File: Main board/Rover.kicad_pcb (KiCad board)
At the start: 2 copper layers, 76.1 x 102.6 mm, 12 parts, among them J1 IN, J2 OUT, J3 Barrel_Jack_Switch, J4 MOTOR, J5 MOTOR, J6 MOTOR, J7 MOTOR, SW1 SW_DPDT_x2, U1 RASPBERRY_PI_4B_4GB

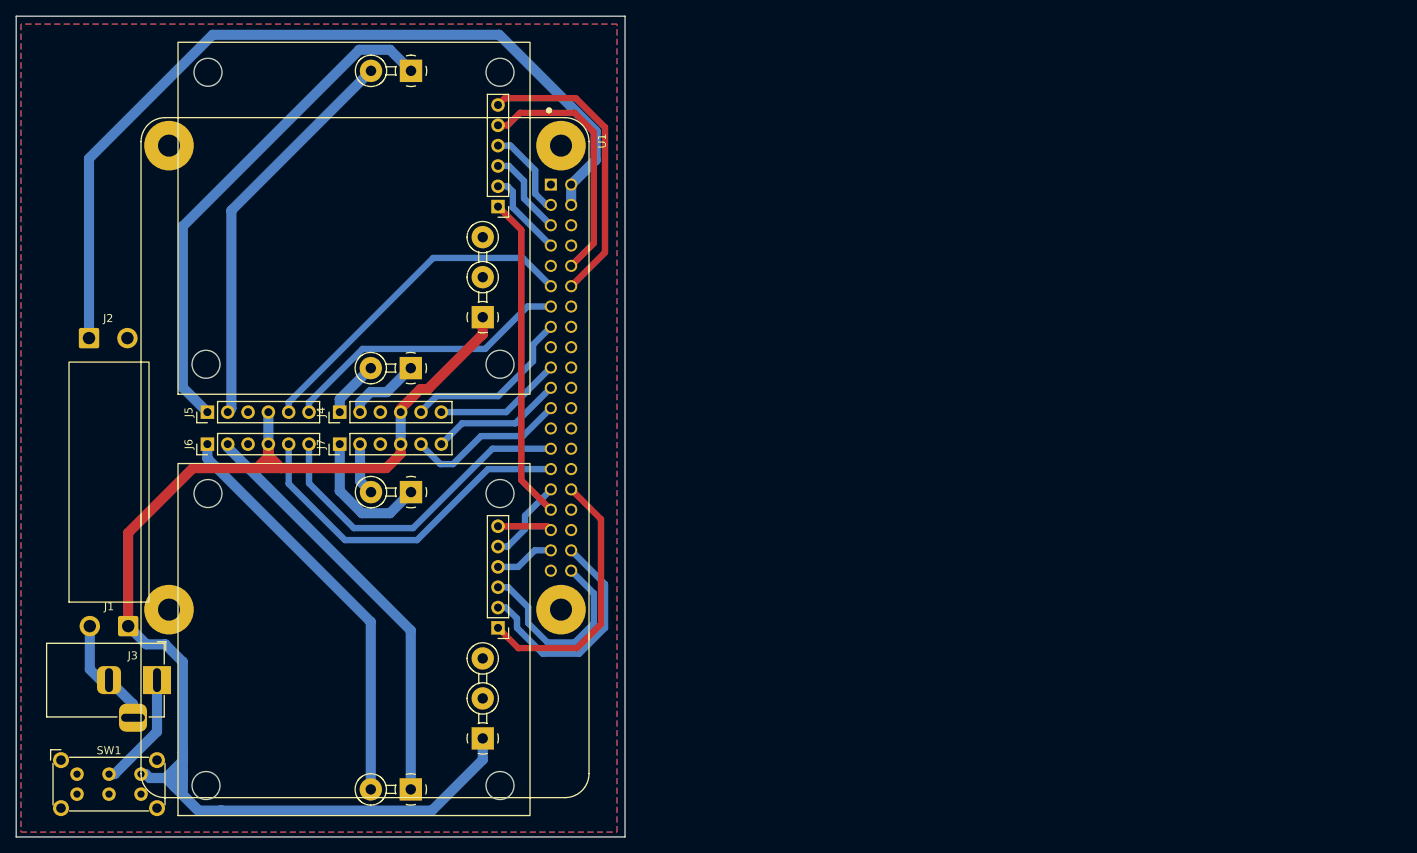
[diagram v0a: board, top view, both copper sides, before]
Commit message: updated pcb
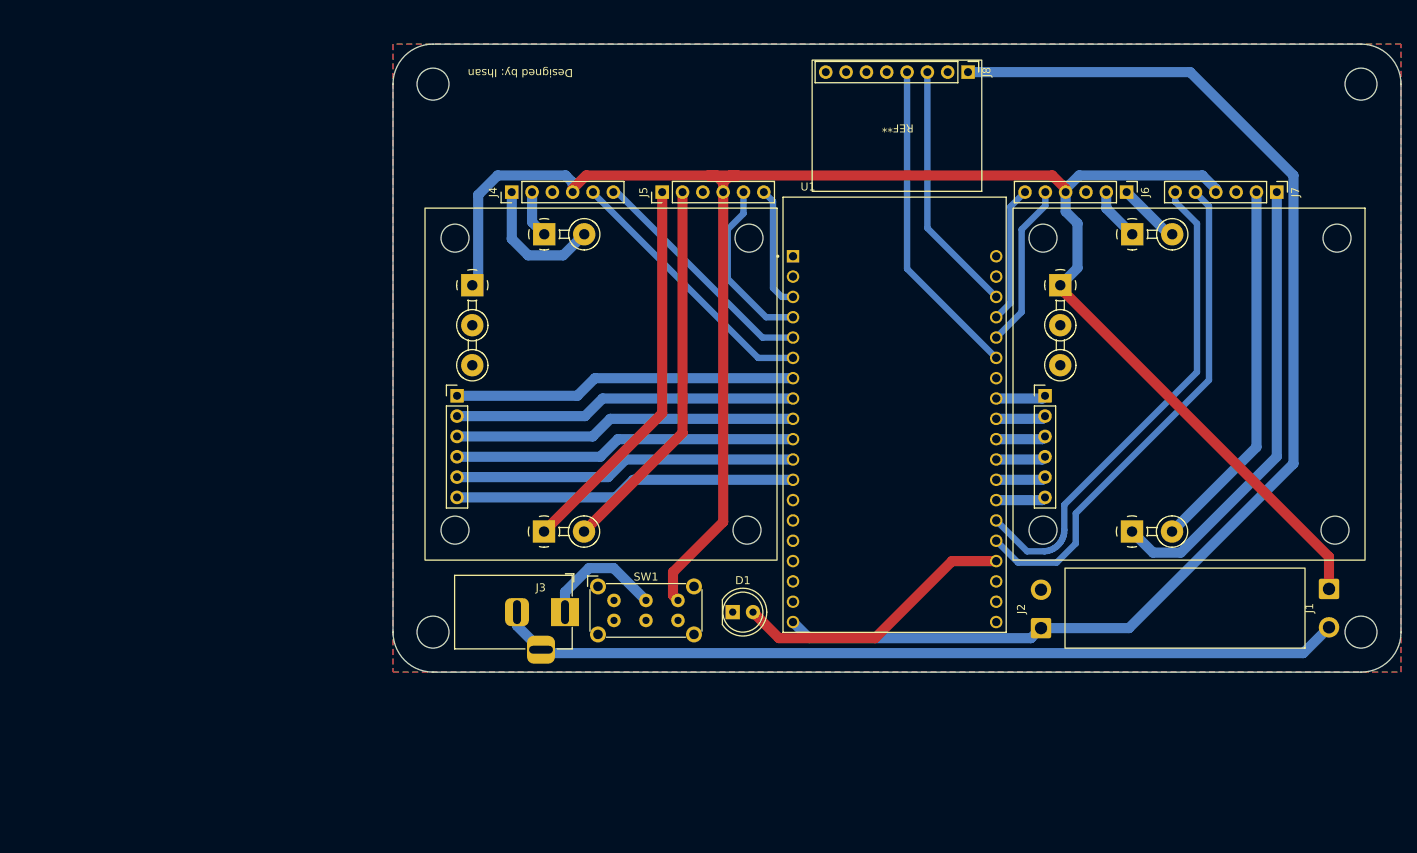
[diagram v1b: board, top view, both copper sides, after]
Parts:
- added D1: LED, LED_THT:LED_D5.0mm_Clear, F.Cu at (178.5, 120.5)
- added J8: IMU, Connector_PinHeader_2.54mm:PinHeader_1x08_P2.54mm_Vertical, F.Cu at (207.9, 53.0)
- added REF**: mpu 6050, module:mpu 6050, F.Cu at (199.1, 59.5)
- U1: value RASPBERRY_PI_4B_4GB -> ESP32-DEVKITC-32D; footprint RASPBERRY_PI_4B_4GB:MODULE_RASPBERRY_PI_4B_4GB -> Library:MODULE_ESP32-DEVKITC-32D
- moved J1 150.2 mm to (253.0, 117.6), turned to -90 degrees
- moved REF** 135.4 mm to (235.0, 120.0), turned to 180 degrees
- moved J2 124.4 mm to (217.0, 122.5), turned to 90 degrees
- moved J7 121.3 mm to (246.5, 68.0), turned to -90 degrees
- moved J6 119.1 mm to (227.7, 68.0), turned to -90 degrees
- moved U3 109.1 mm to (235.5, 92.0), turned to -90 degrees
- moved SW1 70.5 mm to (163.6, 119.0)
- moved U1 66.4 mm to (198.7, 95.8), turned to 0 degrees
- moved J5 63.2 mm to (169.7, 68.0)
- moved J3 51.7 mm to (157.5, 120.5)
- moved U2 37.2 mm to (162.0, 92.0), turned to -90 degrees
- moved J4 34.9 mm to (150.8, 68.0)
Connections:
- U2 pad 1: PWM1 -> Net-(U1-IO32)
- U2 pad 2: IN1 1 -> Net-(U1-IO33)
- U2 pad 3: IN2 1 -> Net-(U1-IO25)
- U2 pad 4: IN3 1 -> Net-(U1-IO26)
- U2 pad 5: IN4 1 -> Net-(U1-IO27)
- U2 pad 6: PWM3 -> Net-(U1-IO14)
- U3 pad 1: PWM0 -> Net-(U1-IO19)
- U3 pad 2: IN1 2 -> Net-(U1-IO18)
- U3 pad 3: IN2 2 -> Net-(U1-IO5)
- U3 pad 4: IN3 2 -> Net-(U1-IO17)
- U3 pad 5: IN4 2 -> Net-(U1-IO16)
- U3 pad 6: PWM2 -> Net-(U1-IO4)
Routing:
- net Net-(J1-Pin_2): track 14.3 -> 106.0 mm
- net +7.4V: track 169.7 -> 235.1 mm
- net +5V: track 107.7 -> 154.5 mm
- net Net-(J6-Pin_2): track 52.6 -> 6.61 mm
- net SIG B 4: track 16.6 -> 61.9 mm
- net Net-(J6-Pin_1): track 51.6 -> 7.89 mm
- net SIG A 4: track 20.2 -> 63.6 mm
- net Net-(U1-IO33): track 0.00 -> 42.9 mm
- net Net-(U1-IO25): track 0.00 -> 42.9 mm
- net Net-(U1-IO14): track 0.00 -> 42.9 mm
- net Net-(U1-IO27): track 0.00 -> 42.9 mm
- net Net-(U1-IO26): track 0.00 -> 42.9 mm
- net Net-(U1-IO32): track 0.00 -> 42.9 mm
- net PWM1: track 40.6 -> 0.00 mm
- net Net-(J8-Pin_4): track 0.00 -> 40.3 mm
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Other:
- board size 76.1 x 102.6 mm -> 126 x 78.5 mm
- board text added: "Designed by: Ihsan"
